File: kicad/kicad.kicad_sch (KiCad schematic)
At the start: 70 parts, among them P1 RZM001P02T2L, P10 RZM001P02T2L, P11 RZM001P02T2L, P12 RZM001P02T2L, P13 RZM001P02T2L, P14 RZM001P02T2L, P15 RZM001P02T2L, P16 RZM001P02T2L, P17 RZM001P02T2L, P18 RZM001P02T2L, P19 RZM001P02T2L, P2 RZM001P02T2L, P20 RZM001P02T2L, P21 RZM001P02T2L, P22 RZM001P02T2L, P23 RZM001P02T2L, P24 RZM001P02T2L, P25 RZM001P02T2L, P26 RZM001P02T2L, P27 RZM001P02T2L, P28 RZM001P02T2L, P29 RZM001P02T2L, P3 RZM001P02T2L, P30 RZM001P02T2L, P31 RZM001P02T2L, P4 RZM001P02T2L, P5 RZM001P02T2L, P6 RZM001P02T2L, P7 RZM001P02T2L, P8 RZM001P02T2L, P9 RZM001P02T2L

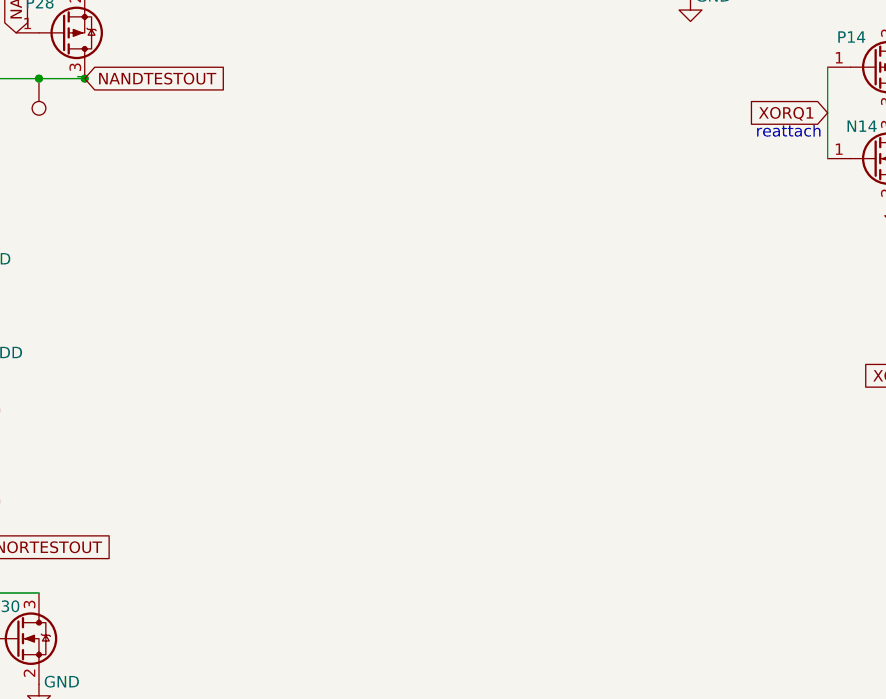
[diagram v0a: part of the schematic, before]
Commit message: More wacky circuits
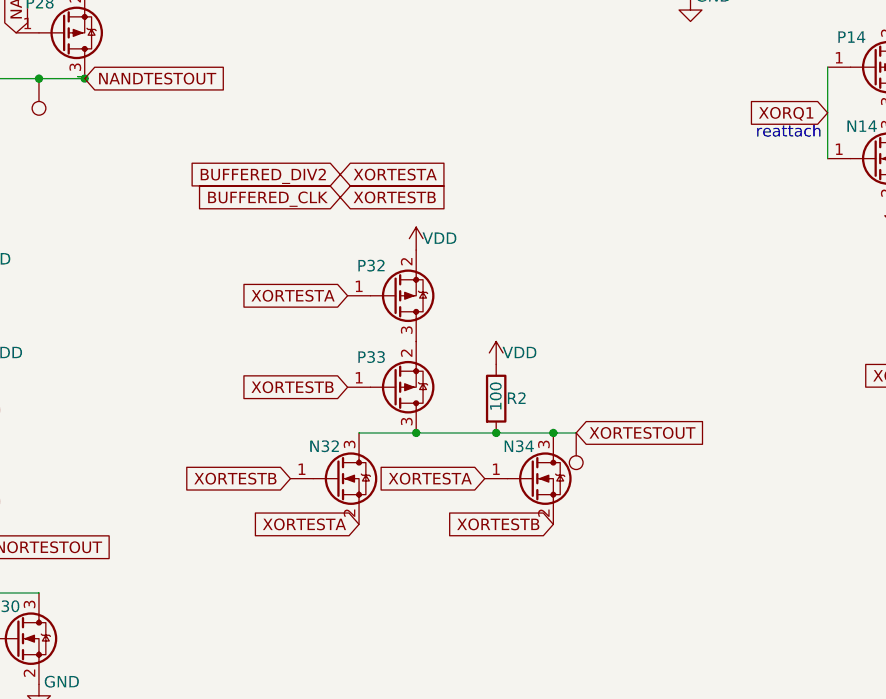
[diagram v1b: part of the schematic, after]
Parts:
- added N32, N34: 2SK3541, cnhardware:SOT-723-COMPACT, symbol Device:Q_NMOS_GSD
- added P32, P33: RZM001P02T2L, cnhardware:SOT-723-COMPACTP, symbol Device:Q_PMOS_GSD
- added R2: 100, cnhardware:R_0402_1005Metric_COMPACT, symbol Device:R
- added TP3: TP, cnhardware:TPTHRU, symbol Connector:TestPoint
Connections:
- net BUFFERED_CLK: now also N32.1 (G), N34.2 (S), P33.1 (G)
- net BUFFERED_DIV2: now also N32.2 (S), N34.1 (G), P32.1 (G)
- net VDD: now also P32.2 (S), R2.1
- new net: P32.3 (D), P33.2 (S)
- new net XORTESTOUT: N32.3 (D), N34.3 (D), P33.3 (D), R2.2, TP3.1
